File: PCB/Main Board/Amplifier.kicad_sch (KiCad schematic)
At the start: 33 parts, among them U1 DG411xY

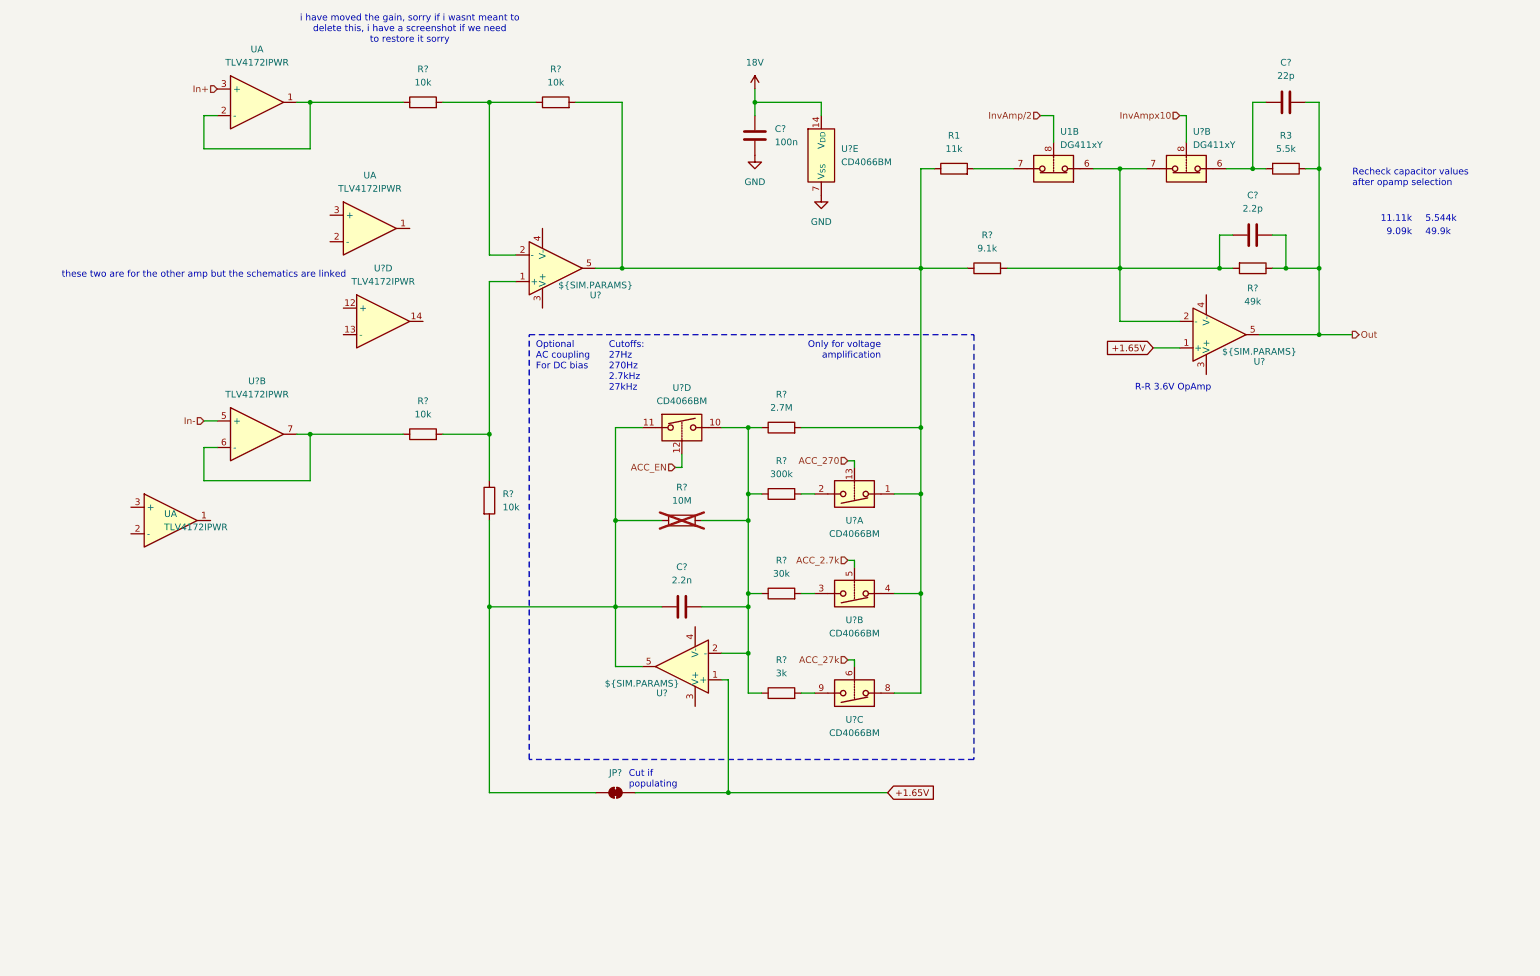
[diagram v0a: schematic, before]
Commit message: :anguished:
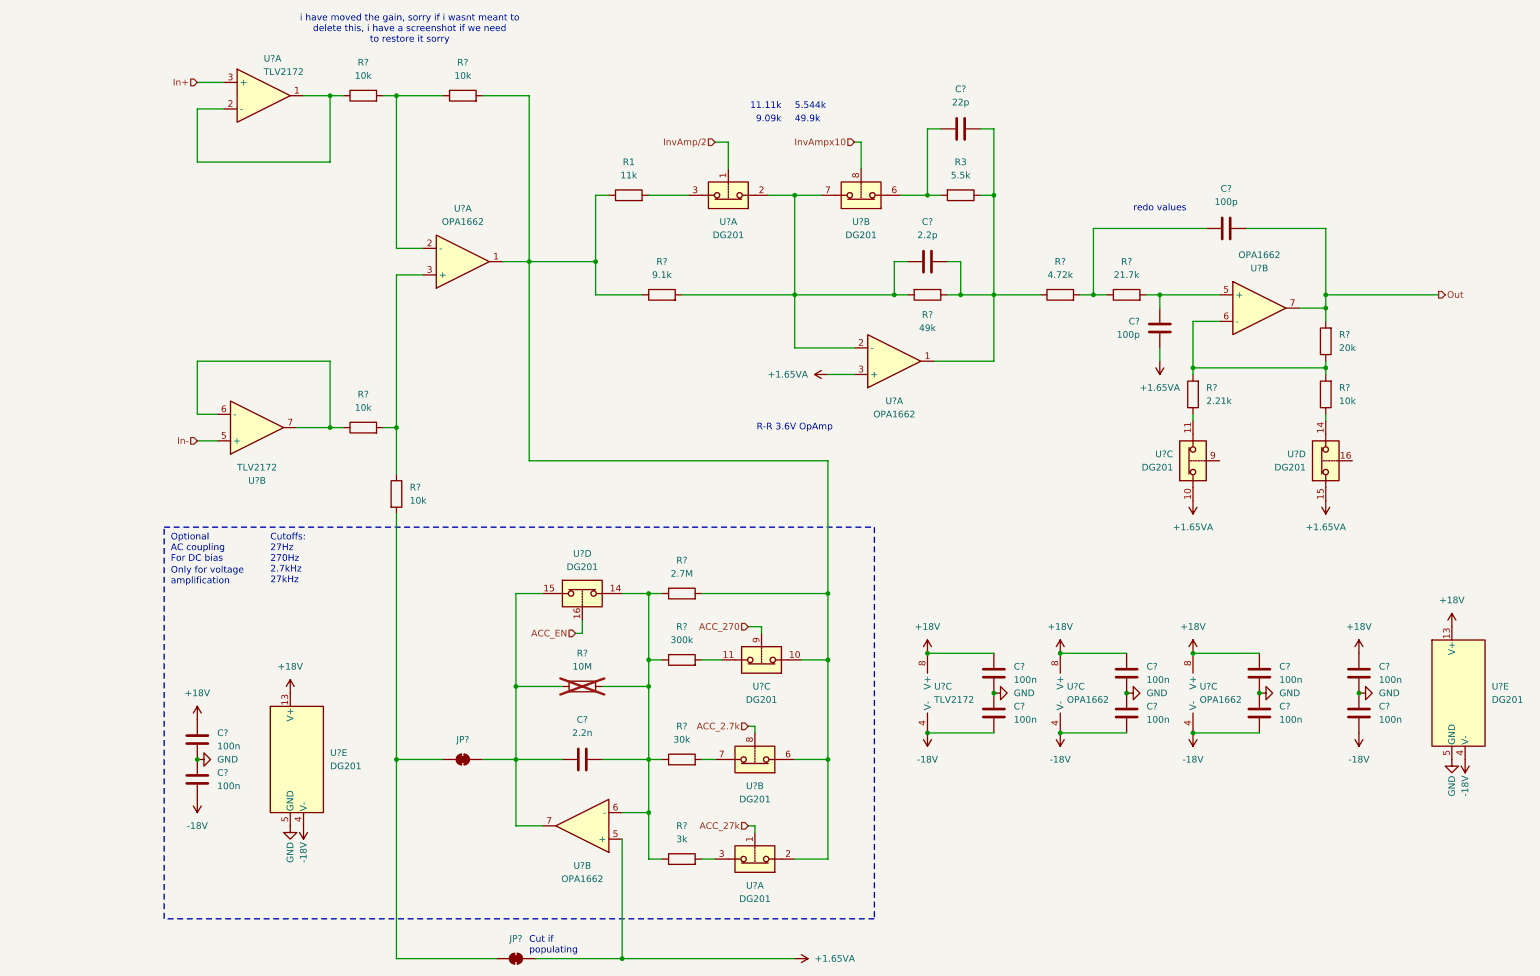
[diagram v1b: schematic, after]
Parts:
- removed C?: 100n, symbol Device:C
- removed U (x3), U? (x2): TLV4172IPWR, symbol Device:Opamp_Quad
- removed U1, U?: DG411xY, Package_SO:SOIC-16_3.9x9.9mm_P1.27mm, symbol Analog_Switch:DG411xY
- removed U? (x5): CD4066BM, Package_SO:SO-14_3.9x8.65mm_P1.27mm, symbol Analog_Switch:CD4066BM
- removed U? (x3): ${SIM.PARAMS}, symbol Simulation_SPICE:OPAMP
- added C? (x10): 100n, symbol Device:C
- added C? (x2): 100p, symbol Device:C
- added JP?: SolderJumper_2_Bridged, Jumper:SolderJumper-2_P1.3mm_Bridged_RoundedPad1.0x1.5mm, symbol Jumper:SolderJumper_2_Bridged
- added R?: 20k, symbol Device:R
- added R?: 10k, symbol Device:R
- added R?: 2.21k, symbol Device:R
- added R?: 21.7k, symbol Device:R
- added R?: 4.72k, symbol Device:R
- added U? (x10): DG201, Package_SO:SOIC-16_3.9x9.9mm_P1.27mm, symbol More_symbols:DG201
- added U? (x6): OPA1662, Package_SO:SOIC-8_3.9x4.9mm_P1.27mm, symbol Device:Opamp_Dual
- added U? (x3): TLV2172, Package_SO:SOIC-8_3.9x4.9mm_P1.27mm, symbol Device:Opamp_Dual
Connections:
- net ACC_2.7k: now also U?.8
- net ACC_270: now also U?.9
- net ACC_27k: now also U?.1
- net ACC_EN: now also U?.16
- net GND: now also C?.1, C?.1, C?.1, C?.1, C?.1, C?.2, C?.2, C?.2, C?.2, C?.2, U?.5 (GND), U?.5 (GND)
- net In+: now also U?.3 (+)
- net In-: now also U?.5 (+)
- net InvAmpx10: now also U?.8
- net InvAmp/2: now also U?.1
- net Out: now also C?.2, R?.2, U?.7; no longer C?.2, C?.2, R3.1, R?.1
- net at R?.1: now also U?.6 (-), U?.7
- net at C?.1, R?.2, R?.2: now also U?.2, U?.2 (-), U?.7
- net at R1.2: now also U?.3
- net at C?.2, R?.1, R?.1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: now also U?.14, U?.6 (-)
- net at R?.2: now also U?.11
- net at R1.1, R?.1, R?.2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: now also U?.1, U?.10, U?.2, U?.6
- net at R?.2: now also U?.3
- net at R?.1, R?.2: now also U?.3 (+)
- net at C?.1, R?.1: now also JP?.2 (B), U?.15, U?.7; no longer JP?.1 (A), R?.2
- net at R?.2: now also U?.7
- net at C?.1, R3.2: now also U?.6
- net at R?.1: now also U?.1, U?.2 (-)
- net at R?.1, R?.2: now also U?.2 (-)
- net +1.65V renamed +1.65VA
- net +1.65VA: now also C?.2, U?.10, U?.15, U?.3 (+), U?.5 (+)
- new net: C?.2, C?.2, R3.1, R?.1, R?.1, U?.1
- new net: R?.1, R?.2, R?.2, U?.6 (-)
- new net: R?.1, U?.14
- new net: JP?.1 (A), JP?.1 (A), R?.2
- new net: R?.1, U?.11
- new net: C?.1, R?.1, R?.2
- new net: C?.1, R?.2, U?.5 (+)
- new net +18V: C?.1, C?.1, C?.1, C?.1, C?.1, U?.13 (V+), U?.13 (V+), U?.8 (V+), U?.8 (V+), U?.8 (V+)
- new net -18V: C?.2, C?.2, C?.2, C?.2, C?.2, U?.4 (V-), U?.4 (V-), U?.4 (V-), U?.4 (V-), U?.4 (V-)
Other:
- note added: "redo values"
- note removed: "Recheck capacitor values after opamp selection"
- note removed: "these two are for the other amp but the schematics are linked"
- moved on the sheet: C?, JP?, R1, R3, R?
